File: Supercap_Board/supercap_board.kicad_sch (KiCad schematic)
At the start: 4 parts

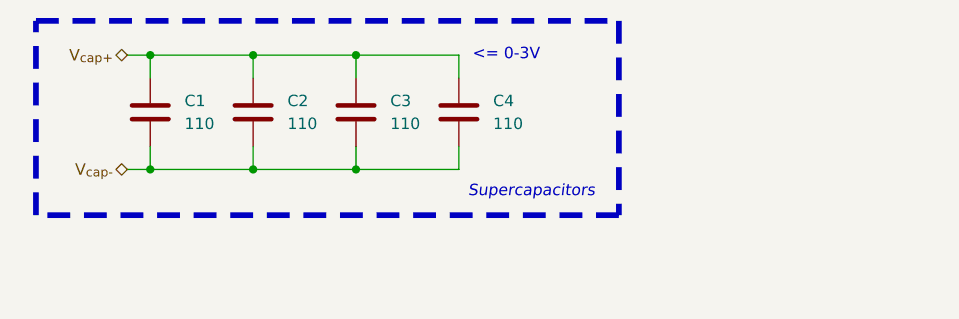
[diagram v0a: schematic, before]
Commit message: big progress on layout
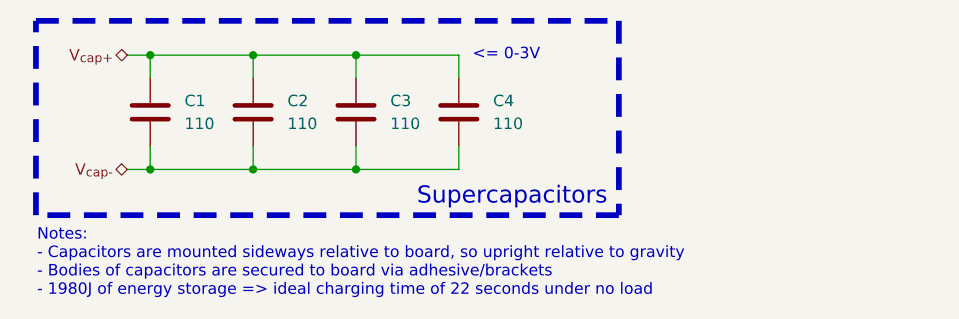
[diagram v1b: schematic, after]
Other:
- note added: "Notes: - Capacitors are mounted sideways relative to board, so upright relative to gravity - Bodies of capacitors are secured to board via adhesive/brackets - 1980J of energy storage => ideal charging time of 22 seconds under no load"
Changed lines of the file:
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@@
+		)
+	)
+	(text "Notes:\n- Capacitors are mounted sideways relative to board, so upright relative to gravity\n- Bodies of capacitors are secured to board via adhesive/brackets\n- 1980J of energy storage => ideal charging time of 22 seconds under no load"
+		(exclude_from_sim no)
+		(at 73.787 78.994 0)
+		(effects
+			(font
+				(size 1.27 1.27)
+			)
+			(justify left)
+		)
+	)
+	(text "Supercapacitors"
+		(exclude_from_sim no)
+		(at 137.16 71.628 0)
+		(effects
+			(font
+				(size 1.905 1.905)
+			)
+			(justify right)
 		)
 	)
@@
 		)
 	)
-	(text "Supercapacitors"
-		(exclude_from_sim no)
-		(at 121.666 70.358 0)
-		(effects
-			(font
-				(size 1.27 1.27)
-				(italic yes)
-			)
-			(justify left top)
-		)
-	)
